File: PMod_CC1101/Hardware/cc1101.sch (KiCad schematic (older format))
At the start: 18 parts, among them J1 Conn_Coaxial, J2 Conn_02x06_Odd_Even, U1 CC1101RGPR

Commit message: initial footprint for the CC1101 part
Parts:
- U1: footprint (none) -> Package_DFN_QFN:UQFN-20-1EP_4x4mm_P0.5mm_EP2.8x2.8mm
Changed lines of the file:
@@
 F 0 "U1" H 4575 2315 50  0000 C CNN
 F 1 "CC1101RGPR" H 4575 2224 50  0000 C CNN
-F 2 "" H 4250 1900 50  0001 C CNN
+F 2 "Package_DFN_QFN:UQFN-20-1EP_4x4mm_P0.5mm_EP2.8x2.8mm" H 4250 1900 50  0001 C CNN
 F 3 "" H 4250 1900 50  0001 C CNN
 	1    4600 1900

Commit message: add footprint missing on cap
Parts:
- C131: footprint (none) -> Capacitor_SMD:C_0603_1608Metric
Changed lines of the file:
@@
 F 0 "C131" H 6515 2146 50  0000 L CNN
 F 1 "3.9pF" H 6515 2055 50  0000 L CNN
-F 2 "" H 6438 1950 50  0001 C CNN
+F 2 "Capacitor_SMD:C_0603_1608Metric" H 6438 1950 50  0001 C CNN
 F 3 "~" H 6400 2100 50  0001 C CNN
 	1    6400 2100

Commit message: update schematic part for cc1101
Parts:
- U1: footprint Package_DFN_QFN:UQFN-20-1EP_4x4mm_P0.5mm_EP2.8x2.8mm -> jjh:QFN50P400X400X100-21N-D
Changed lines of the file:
@@
 F 0 "U1" H 4575 2315 50  0000 C CNN
 F 1 "CC1101RGPR" H 4575 2224 50  0000 C CNN
-F 2 "Package_DFN_QFN:UQFN-20-1EP_4x4mm_P0.5mm_EP2.8x2.8mm" H 4250 1900 50  0001 C CNN
+F 2 "jjh:QFN50P400X400X100-21N-D" H 4250 1900 50  0001 C CNN
 F 3 "" H 4250 1900 50  0001 C CNN
 	1    4600 1900

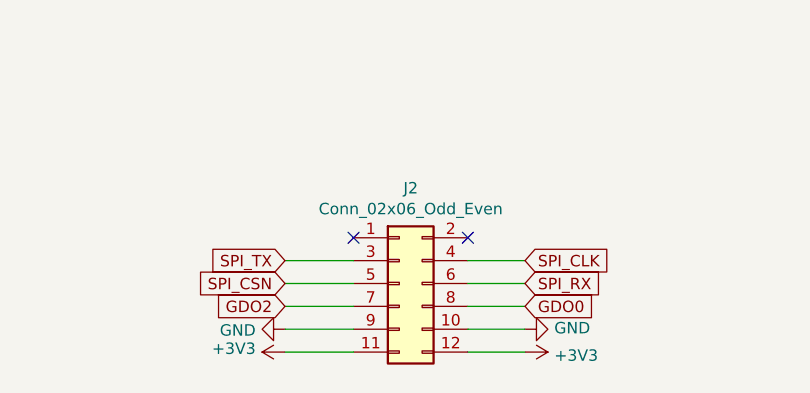
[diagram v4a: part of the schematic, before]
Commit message: Update the connector layout
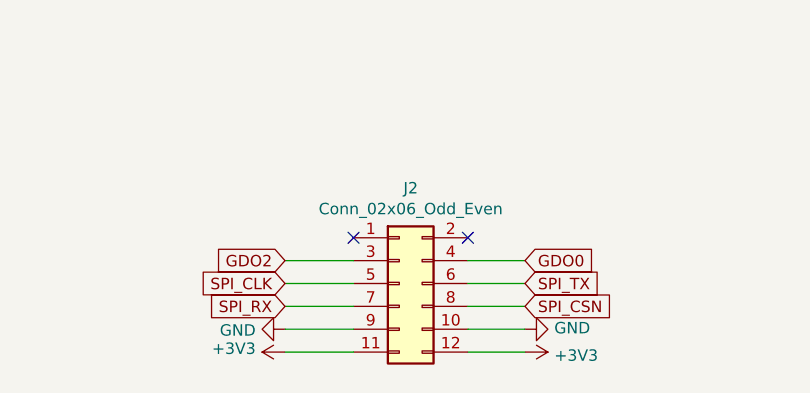
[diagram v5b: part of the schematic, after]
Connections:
- net GDO0: now also J2.4 (Pin_4); no longer J2.8 (Pin_8)
- net GDO2: now also J2.3 (Pin_3); no longer J2.7 (Pin_7)
- net SPI_CLK: now also J2.5 (Pin_5); no longer J2.4 (Pin_4)
- net SPI_CSN: now also J2.8 (Pin_8); no longer J2.5 (Pin_5)
- net SPI_RX: now also J2.7 (Pin_7); no longer J2.6 (Pin_6)
- net SPI_TX: now also J2.6 (Pin_6); no longer J2.3 (Pin_3)
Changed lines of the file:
@@
 	0    1    1    0
 $EndComp
-Text GLabel 3850 6050 2    50   Input ~ 0
+Text GLabel 2800 6150 0    50   Input ~ 0
 SPI_CLK
+Text GLabel 2800 6250 0    50   Input ~ 0
+SPI_RX
+Text GLabel 3850 6250 2    50   Input ~ 0
+SPI_CSN
 Text GLabel 3850 6150 2    50   Input ~ 0
-SPI_RX
-Text GLabel 2800 6150 0    50   Input ~ 0
-SPI_CSN
-Text GLabel 2800 6050 0    50   Input ~ 0
 SPI_TX
 Wire Wire Line
@@
 Wire Wire Line
 	5400 3300 5250 3300
-Text GLabel 2800 6250 0    50   Input ~ 0
+Text GLabel 2800 6050 0    50   Input ~ 0
 GDO2
-Text GLabel 3850 6250 2    50   Input ~ 0
+Text GLabel 3850 6050 2    50   Input ~ 0
 GDO0
 Wire Wire Line
